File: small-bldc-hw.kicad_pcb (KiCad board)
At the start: 2 copper layers, 66.1 x 22.7 mm, 98 parts, among them J1 More IO, J2 TEMP, J3 CONN_01X01, J4 CONN_01X01, J5 CONN_01X01, J6 CAN, J7 I2C, J8 CONN_01X01, J9 CONN_01X01, P2 SWD, Q1 BUK7K13-60E, Q2 BUK7K13-60E, Q3 BUK7K13-60E, U1 STM32F042C6T6, U2 AZ1117C, U3 DRV8301, U4 MCP2562-E/SN, Y1 16MHz

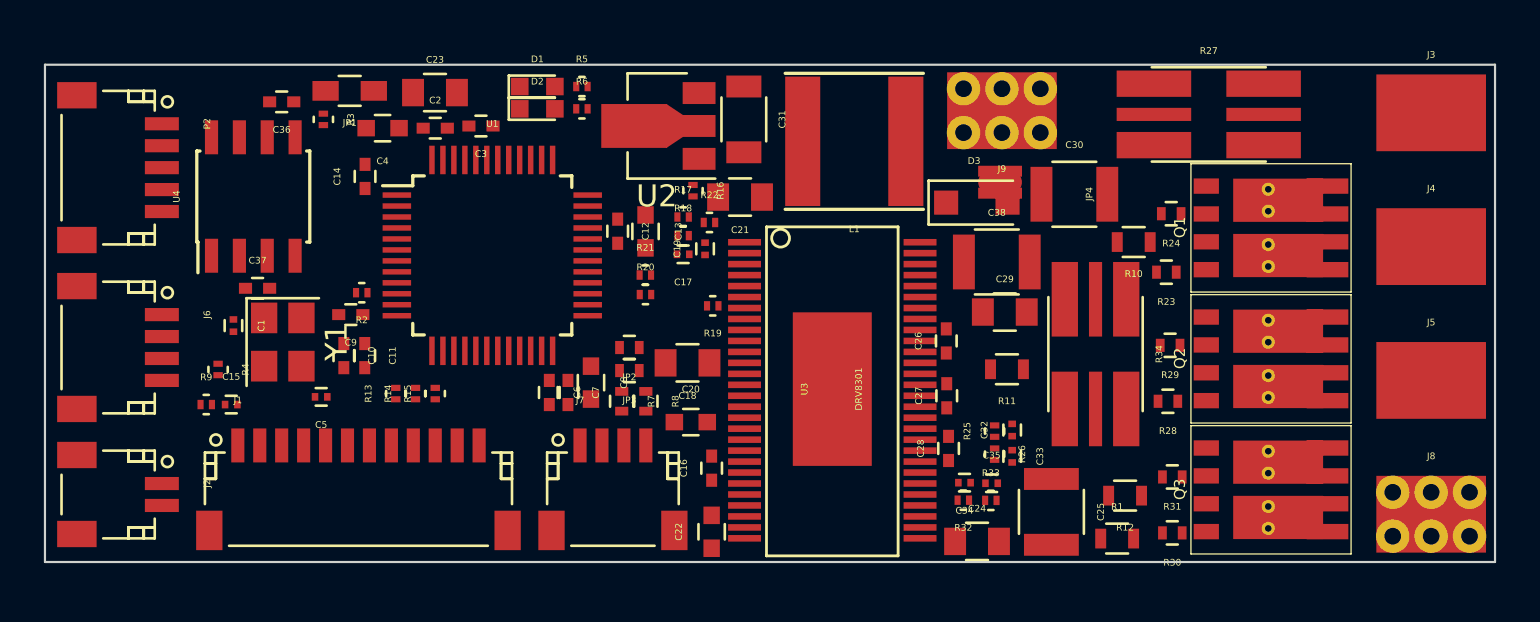
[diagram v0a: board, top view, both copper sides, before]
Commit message: stuff
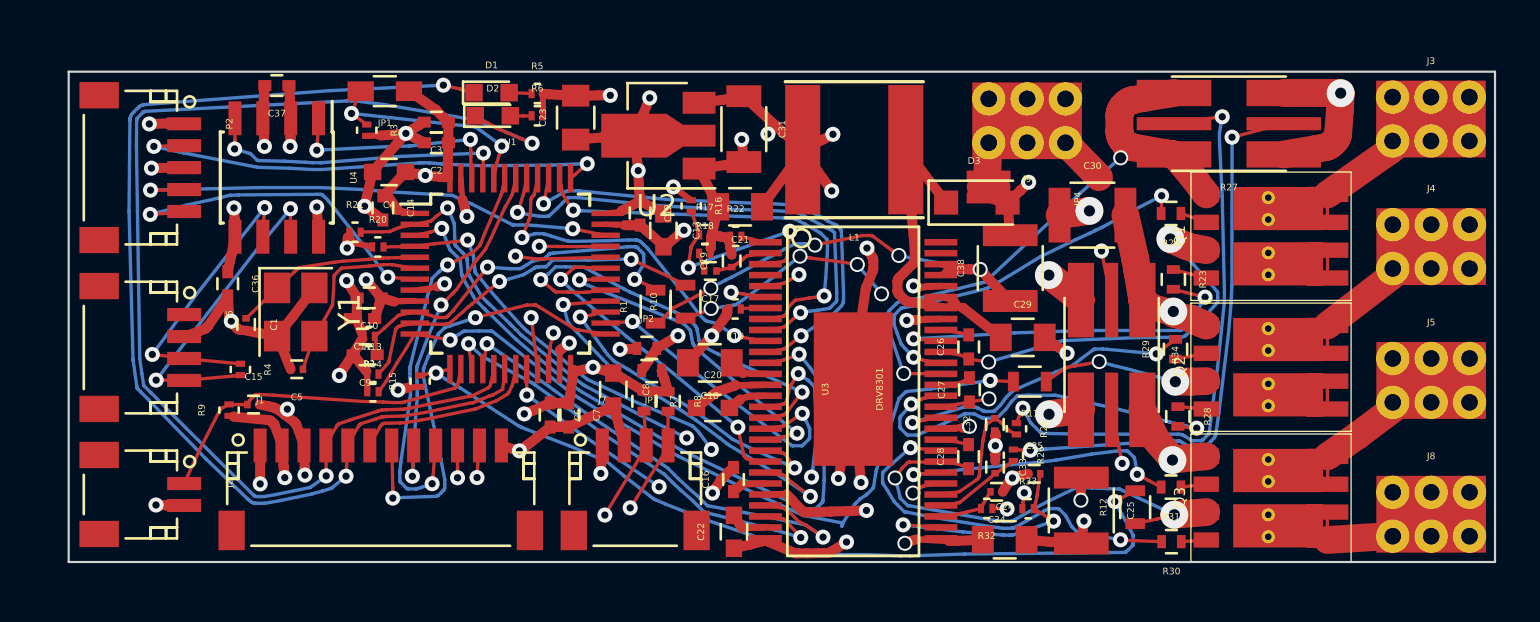
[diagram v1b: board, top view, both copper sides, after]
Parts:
- J3, J4, J5: footprint hlib:SolderWirePad_single_SMD_5x3.5mm -> hlib:SolderWirePad_single_SMD_5x3.5mm_holes
- moved R1 23.5 mm to (146.6, 100.4), turned to 90 degrees
- moved R10 20.6 mm to (148.0, 100.2), turned to 90 degrees
- moved R21 13.4 mm to (132.9, 97.0)
- moved R20 12.4 mm to (134.0, 97.7)
- moved C37 9.28 mm to (129.4, 90.4), turned to 180 degrees
- moved C36 8.65 mm to (127.1, 99.4), turned to 270 degrees
- moved C23 6.52 mm to (143.0, 91.8), turned to 90 degrees
- moved C10 2.87 mm to (133.6, 100.0), turned to 180 degrees
- moved D1 2.11 mm to (139.2, 90.7)
- moved R6 2.06 mm to (141.3, 91.7)
- moved R5 2.06 mm to (141.3, 90.7)
- moved D2 2.06 mm to (139.2, 91.7)
- moved C3 2.04 mm to (136.6, 92.0)
- moved R3 2.04 mm to (133.5, 92.4)
- moved R2 2.02 mm to (133.6, 101.8)
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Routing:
- net GND: track 0.00 -> 237.7 mm, vias 0 -> 29
- net +3V3: track 0.00 -> 137.4 mm, vias 0 -> 12
- net DC_SUPPLY: track 0.00 -> 113.9 mm, vias 0 -> 7
- net +5V: track 0.00 -> 88.1 mm, vias 0 -> 7
- net GNDPWR: track 0.00 -> 70.0 mm, vias 0 -> 4
- net /power/PHASE_A: track 0.00 -> 55.8 mm, vias 0 -> 6
- net /PA7: track 0.00 -> 54.8 mm, vias 0 -> 2
- net /PB0: track 0.00 -> 50.5 mm, vias 0 -> 2
- net /power/PHASE_C: track 0.00 -> 39.4 mm, vias 0 -> 2
- net /PHC_V: track 0.00 -> 38.7 mm, vias 0 -> 2
- net /DRV_OCTW: track 0.00 -> 37.8 mm, vias 0 -> 3
- net /DRV_FAULT: track 0.00 -> 37.1 mm, vias 0 -> 3
- net /PHB_V: track 0.00 -> 37.1 mm, vias 0 -> 2
- net /DRV_DC_CAL: track 0.00 -> 32.5 mm, vias 0 -> 2
- net /power/PHASE_B: track 0.00 -> 32.3 mm, vias 0 -> 3
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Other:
- board size 66.1 x 22.7 mm -> 65 x 22.4 mm
- copper layers 2 -> 4
- net class Default: clearance 0.15367 -> 0.1524
- net class smallpower: clearance 0.15367 -> 0.1524
- rule trace_clearance: 0.15367 -> 0.1524
- rule trace_min: 0.1524 -> 0
